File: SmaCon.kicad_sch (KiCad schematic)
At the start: 47 parts, among them J1 USB_C_Receptacle, J2 STM32_Debug, J3 Conn_01x03, J4 GT911, J5 ST7789, J6 AudioJack, M1 LD14-002, Q1 AO3400A, SW1 SW_Push, SW2 SW_Push, SW3 SW_Push, SW4 SW_Push, SW5 SW_TMHU27, U1 25LC080C, U2 LXES11DAA2-137, U3 NJM2884U1, U4 BD6211, U5 STM32U575CIUxQ, U6 BD45285, U7 YMF825, Y1 12.288MHz

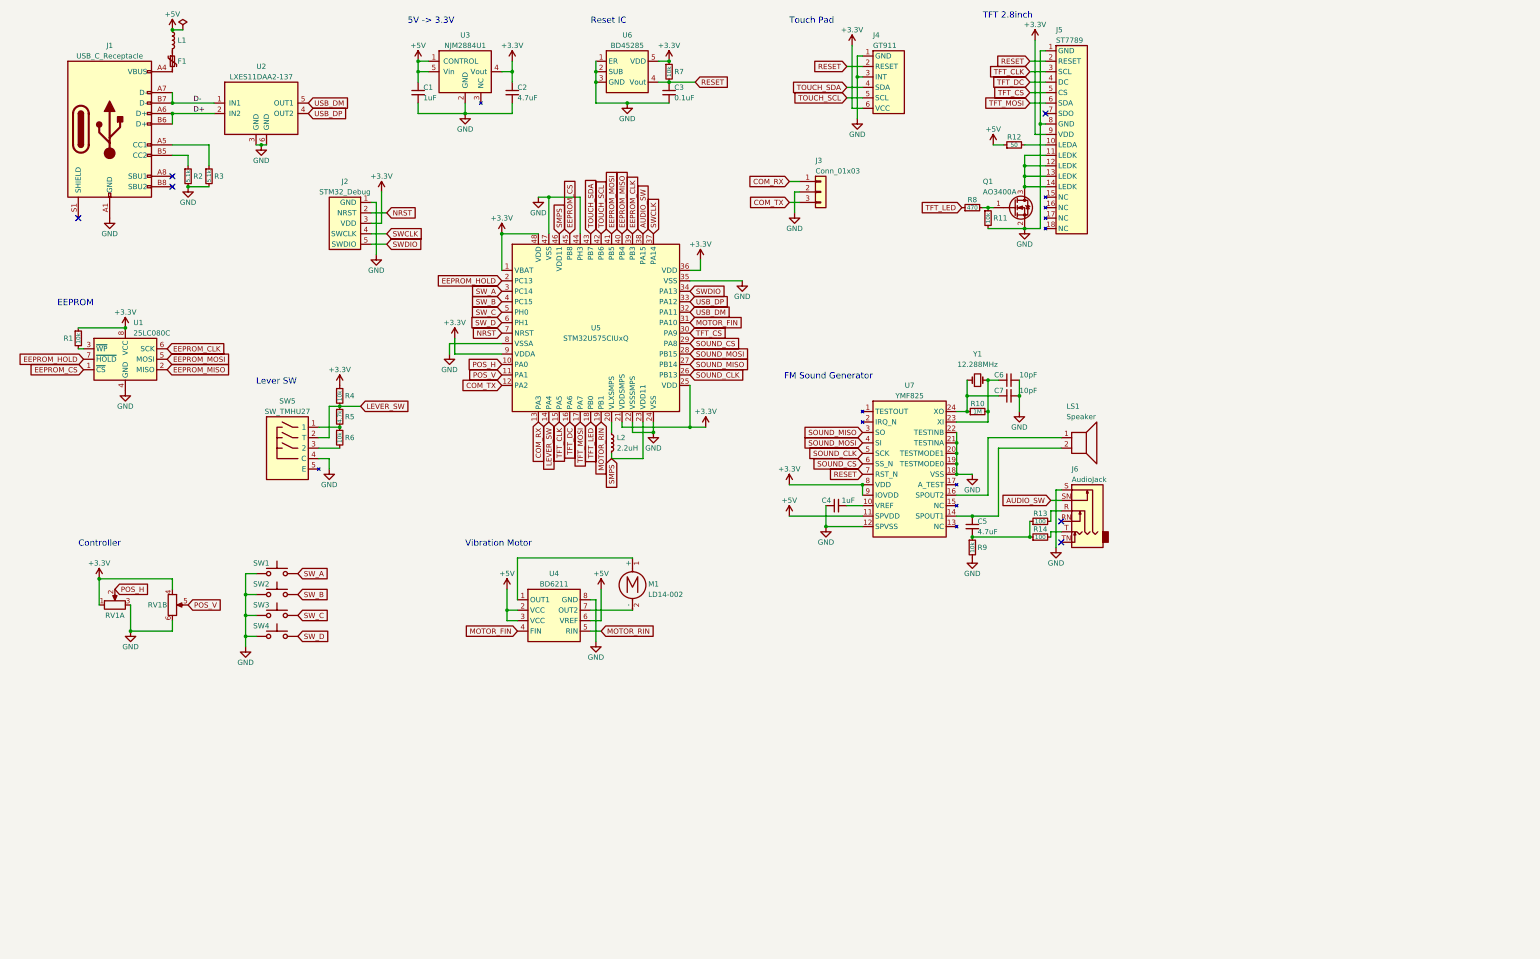
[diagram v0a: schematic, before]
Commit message: 部品選定
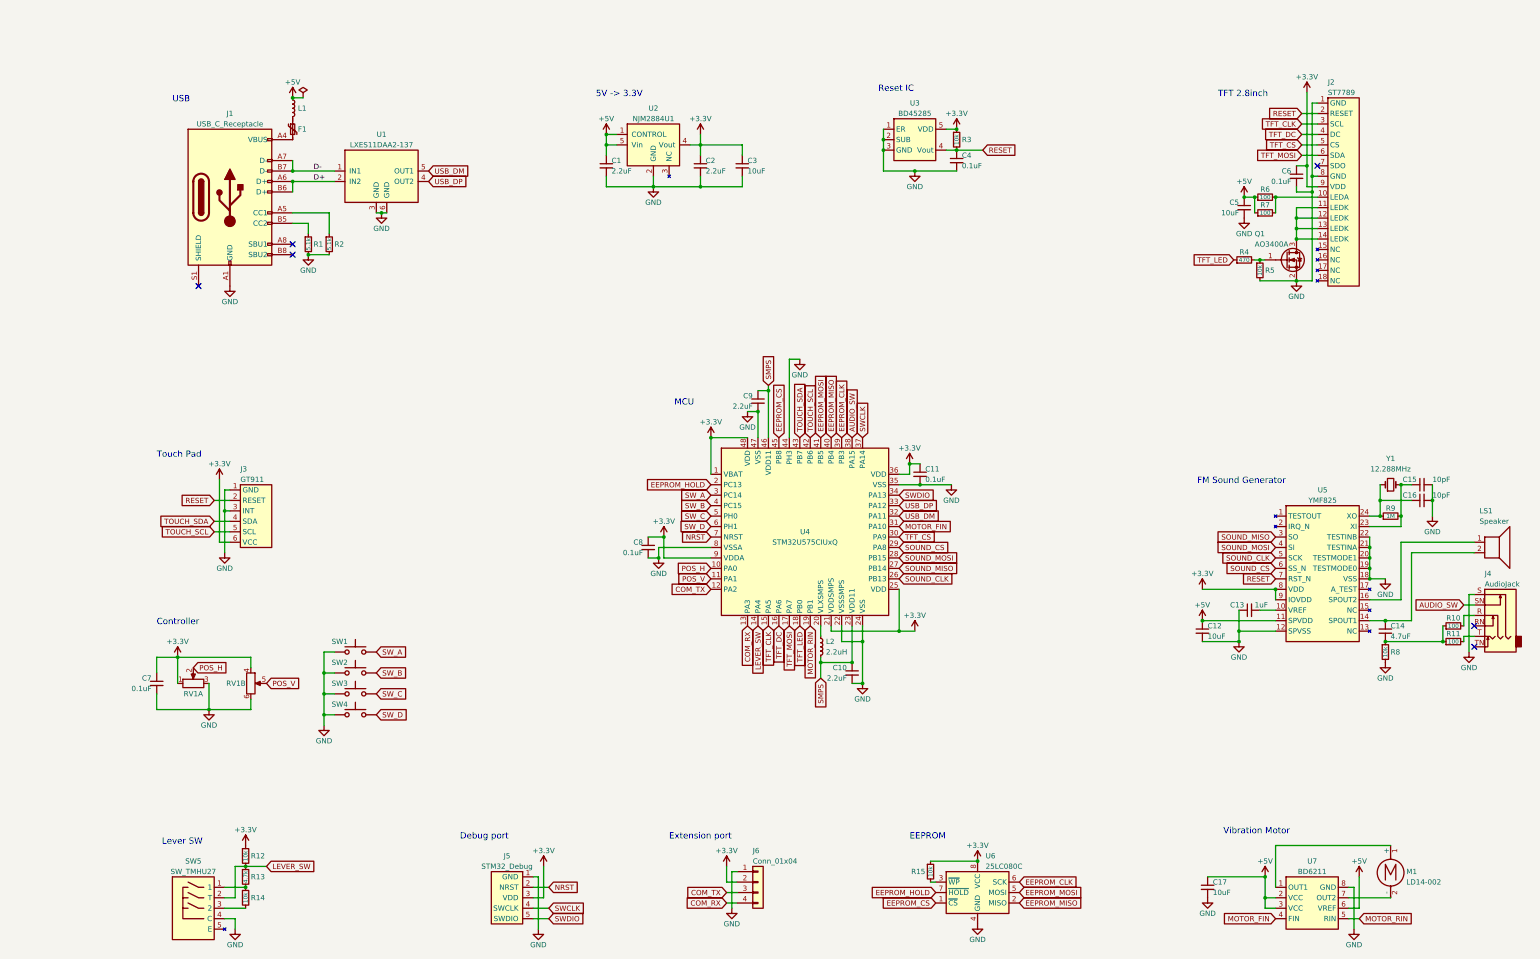
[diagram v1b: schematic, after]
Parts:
- removed J3: Conn_01x03, symbol Connector_Generic:Conn_01x03
- added C10, C9: 2.2uF, SmaCon:1005Metric, symbol Device:C_Small
- added C11, C6, C7, C8: 0.1uF, SmaCon:1005Metric, symbol Device:C_Small
- added C12, C17, C3, C5: 10uF, SmaCon:1608Metric, symbol Device:C_Small
- added J6: Conn_01x04, SmaCon:PinHeader_1x04_P2.54mm_Horizontal, symbol Connector_Generic:Conn_01x04
- added R7: 100, SmaCon:2012Metric, symbol Device:R_Small
- C1: value 1uF -> 2.2uF; footprint (none) -> SmaCon:1005Metric
- C13: renamed from C4; footprint (none) -> SmaCon:1005Metric
- C14: renamed from C5; footprint (none) -> SmaCon:1608Metric
- C15: renamed from C6; footprint (none) -> SmaCon:1005Metric
- C16: renamed from C7; footprint (none) -> SmaCon:1005Metric
- C2: value 4.7uF -> 2.2uF; footprint (none) -> SmaCon:1005Metric
- C4: renamed from C3; footprint (none) -> SmaCon:1005Metric
- F1: footprint (none) -> SmaCon:3216Metric
- J1: footprint (none) -> SmaCon:USB Type-C 5077CR-16SMC2-BK-TR
- J2: renamed from J5; footprint (none) -> SmaCon:Hirose_FH12-18S-0.5SH_1x18-1MP_P0.50mm_Horizontal
- J3: renamed from J4; footprint (none) -> SmaCon:Hirose_FH12-6S-0.5SH_1x06-1MP_P0.50mm_Horizontal
- J4: renamed from J6; footprint (none) -> SmaCon:PJ-3420
- J5: renamed from J2; footprint (none) -> SmaCon:STM32_Debug_5pin
- L1: footprint (none) -> SmaCon:1608Metric
- L2: footprint (none) -> SmaCon:2012Metric
- LS1: footprint (none) -> SmaCon:micro_speaker
- M1: footprint (none) -> SmaCon:LD14-002
- Q1: footprint (none) -> SmaCon:SOT-23
- R1: renamed from R2; footprint (none) -> SmaCon:1005Metric
- R10: renamed from R13; footprint (none) -> SmaCon:2012Metric
- R11: renamed from R14; footprint (none) -> SmaCon:2012Metric
- R12: renamed from R4; footprint (none) -> SmaCon:1005Metric
- R13: renamed from R5; footprint (none) -> SmaCon:1005Metric
- R14: renamed from R6; footprint (none) -> SmaCon:1005Metric
- R15: renamed from R1; footprint (none) -> SmaCon:1005Metric
- R2: renamed from R3; footprint (none) -> SmaCon:1005Metric
- R3: renamed from R7; footprint (none) -> SmaCon:1005Metric
- R4: renamed from R8; footprint (none) -> SmaCon:1005Metric
- R5: renamed from R11; footprint (none) -> SmaCon:1005Metric
- R6: renamed from R12; value 50 -> 100; footprint (none) -> SmaCon:2012Metric
- R8: renamed from R9; footprint (none) -> SmaCon:1005Metric
- R9: renamed from R10; footprint (none) -> SmaCon:1005Metric
- RV1: footprint (none) -> SmaCon:JT8P-3.2T-B10K-1-16Y
- SW1, SW2, SW3, SW4: footprint (none) -> SmaCon:tact_switch
- SW5: footprint (none) -> SmaCon:SW_TMHU27
- U1: renamed from U2; footprint (none) -> SmaCon:LXES11D
- U2: renamed from U3; footprint Package_TO_SOT_SMD:SOT-89-5_Handsoldering -> SmaCon:SOT-89-5
- U3: renamed from U6; footprint (none) -> SmaCon:SOT-23-5
- U4: renamed from U5; footprint (none) -> SmaCon:QFN-48-1EP_7x7mm_P0.5mm_EP5.3x5.3mm
- U5: renamed from U7; footprint (none) -> SmaCon:SSOP-24_5.3x8.2mm_P0.65mm
- U6: renamed from U1; footprint (none) -> SmaCon:MSOP-8_3x3mm_P0.65mm
- U7: renamed from U4; footprint (none) -> SmaCon:SOP-8_4.4x5.0mm_P1.27mm
- Y1: footprint (none) -> SmaCon:Crystal_SMD_TXC_AX_8045-2Pin_8.0x4.5mm
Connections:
- net +3.3V: now also C11.1, C3.1, C6.1, C7.1, C8.1, J6.2 (Pin_2)
- net +5V: now also C12.1, C17.1, C5.1, R7.1
- net COM_RX: now also J6.4 (Pin_4)
- net COM_TX: now also J6.3 (Pin_3)
- net GND: now also C10.2, C11.2, C12.2, C17.2, C3.2, C5.2, C6.2, C7.2, C8.2, C9.2, J6.1 (Pin_1)
- net SMPS: now also C10.1, C9.1
- net at J2.10 (LEDA), R6.2: now also R7.2
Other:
- note added: "Debug port"
- note added: "Extension port"
- note added: "MCU"
- note added: "USB"
- moved on the sheet: C1, C13, C14, C15, C16, C2, C4, F1, J1, J2, J3, J4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
